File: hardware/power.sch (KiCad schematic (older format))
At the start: 45 parts, among them U200 SY8089AAC, U220 SY8089AAC, U230 SY8089AAC, U250 TPS62088_FIXED, U255 LM3281, U260 NCP707_XDFN4

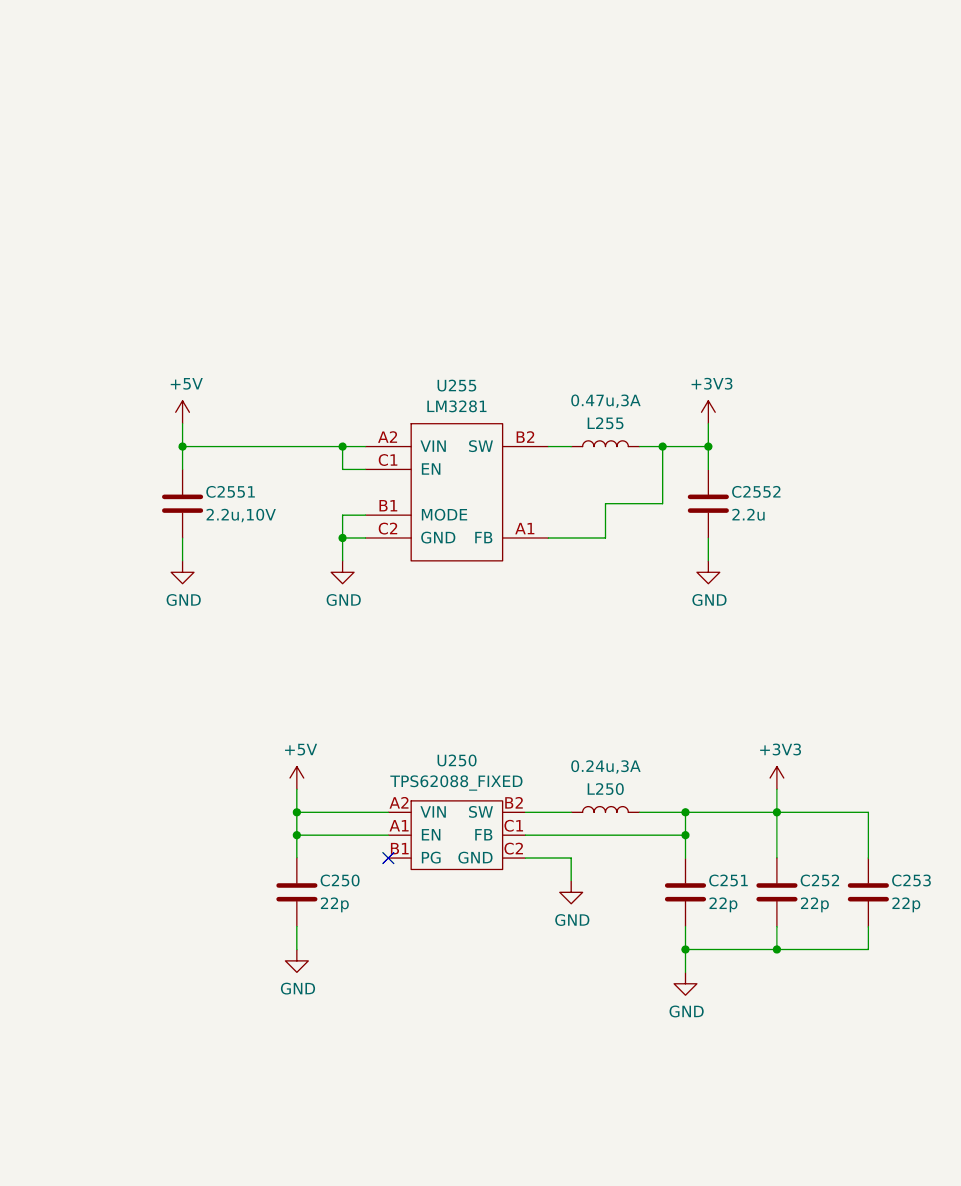
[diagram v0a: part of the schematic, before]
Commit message: wip
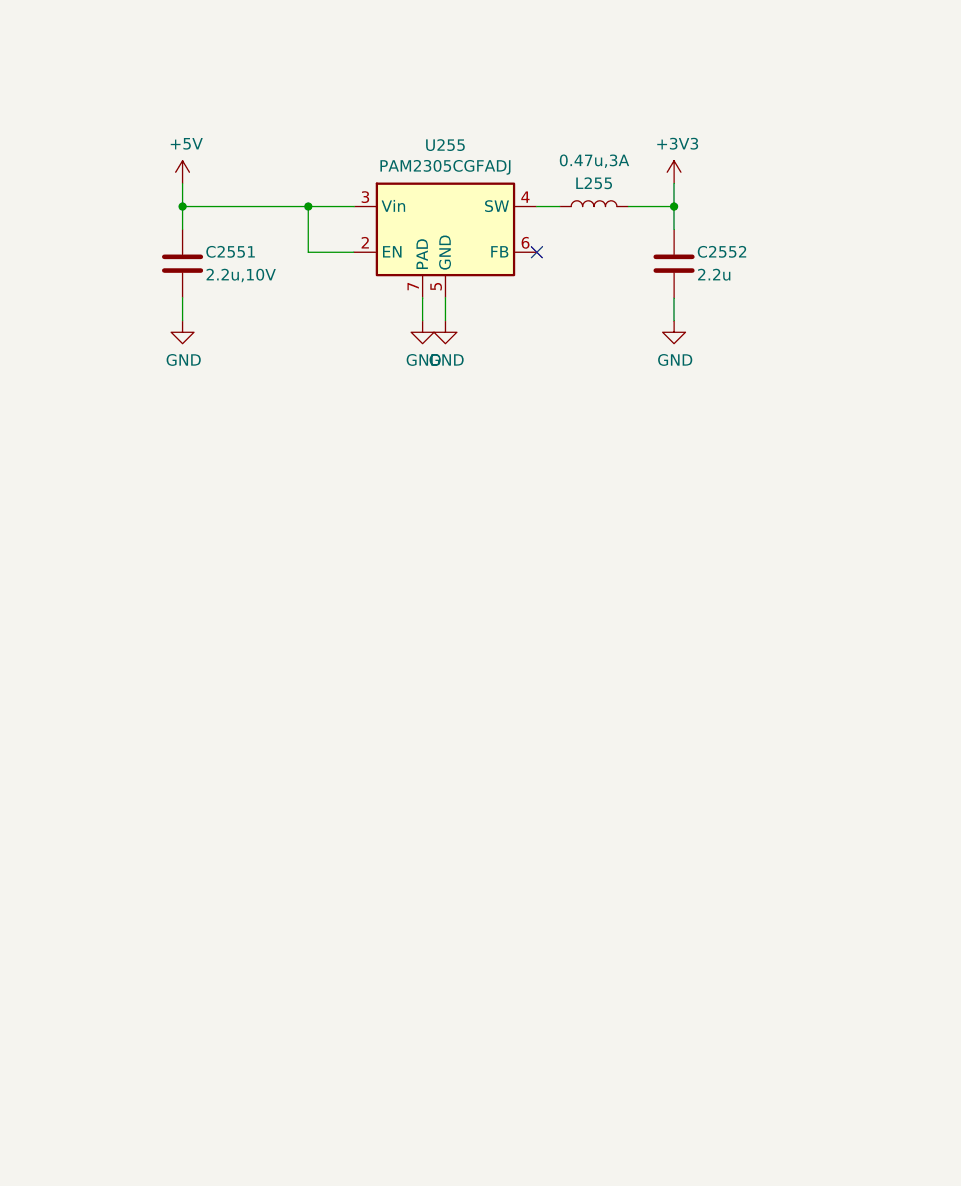
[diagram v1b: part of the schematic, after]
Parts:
- removed C250, C252, C253: 22p, require:C_0402, symbol require-rescue:C
- removed C251: 22p, require:C_0402, symbol Device:C
- removed L250: 0.24u,3A, Inductors_SMD:L_0603, symbol Device:L
- removed U250: TPS62088_FIXED, require:TPS62088_DSBGA6, symbol require:TPS62088_FIXED
- removed U255: LM3281, require:LM3281_DSBGA6, symbol require:LM3281
- added U255: PAM2305CGFADJ, require:U-DFN2020-6, symbol Regulator_Switching:PAM2305CGFADJ
- C2551, C2552: footprint require:C_0402 -> require:C_0603
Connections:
- net +5V: now also U255.2 (EN), U255.3 (Vin)
- net GND: now also U255.5 (GND), U255.7 (PAD)
- net at L255.1: now also U255.4 (SW)
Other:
- moved on the sheet: C2551, C2552, L255
